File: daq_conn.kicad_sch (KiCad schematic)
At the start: 1 part

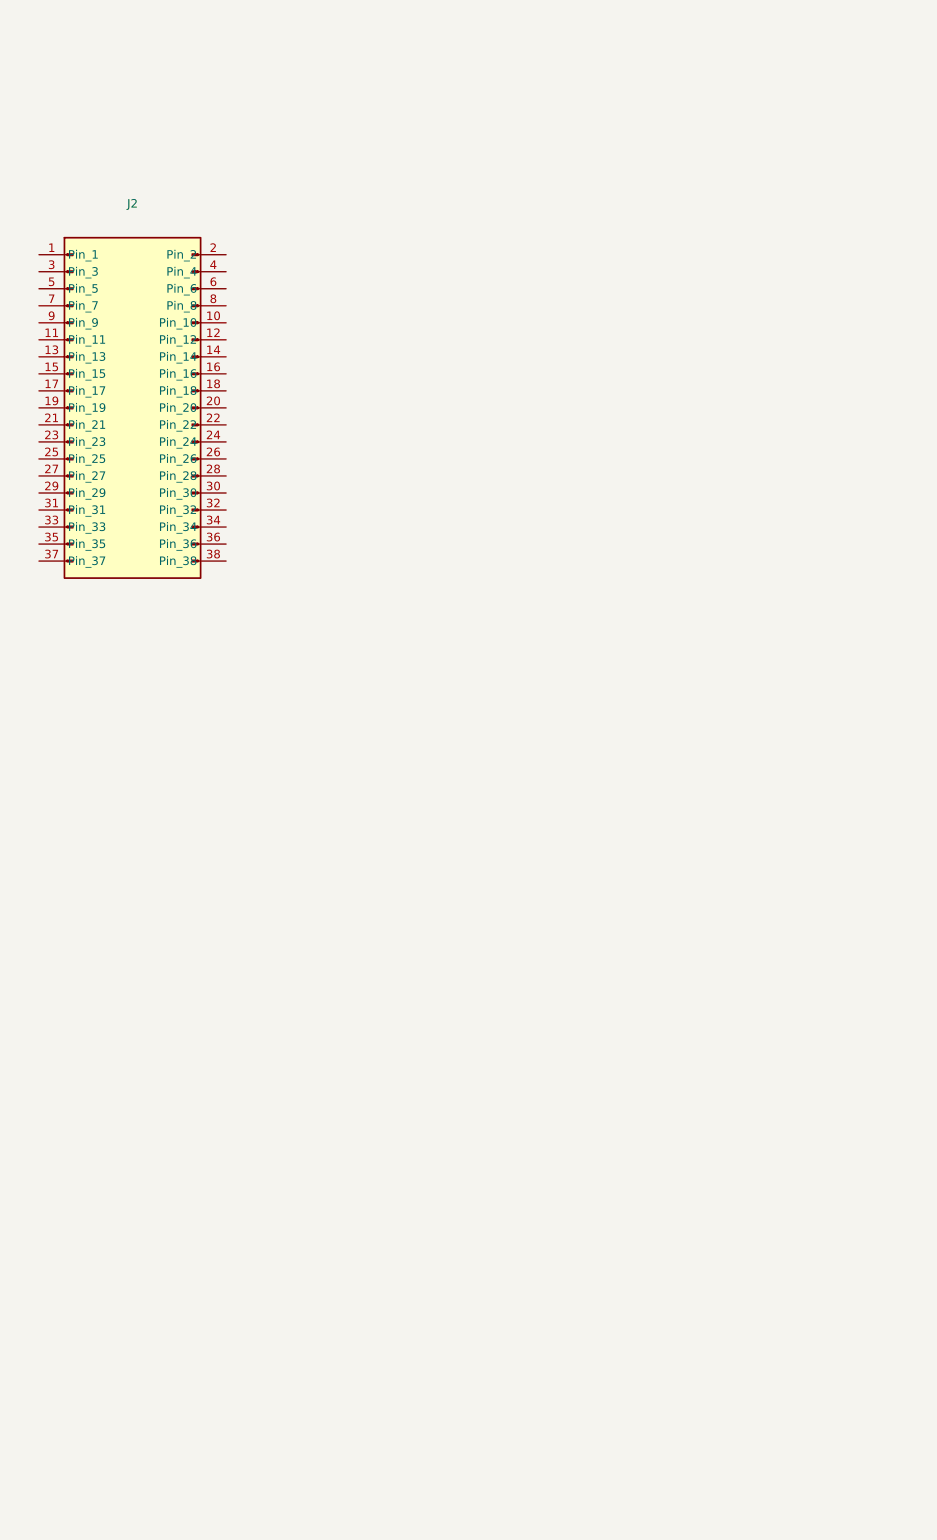
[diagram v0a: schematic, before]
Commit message: started on adc
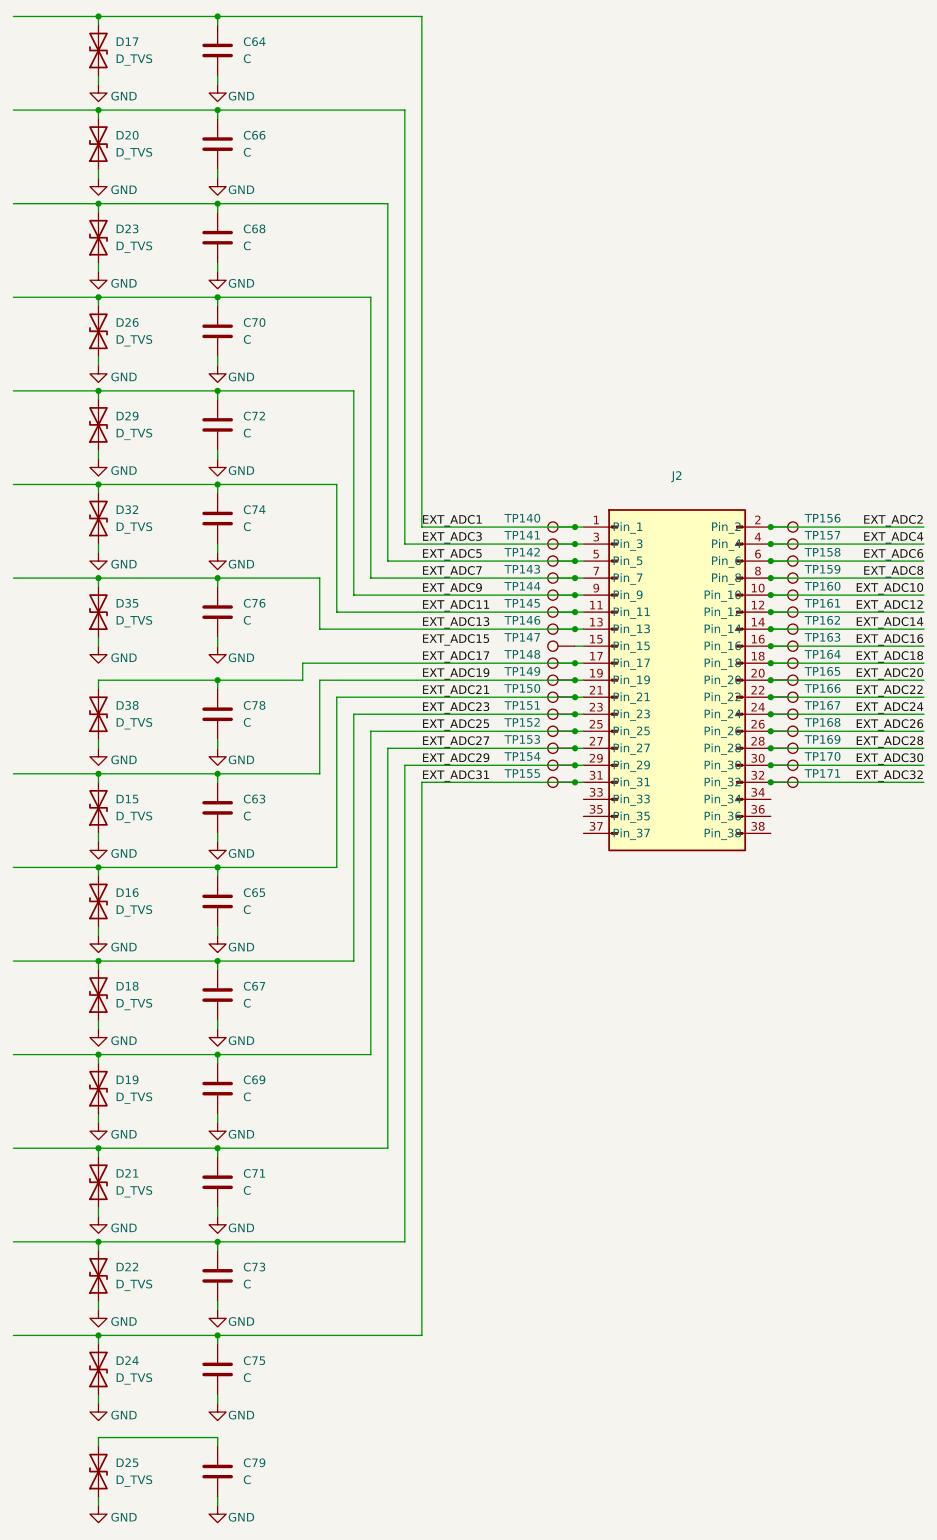
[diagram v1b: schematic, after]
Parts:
- added C63, C64, C65, C66, C67, C68, C69, C70, C71, C72, C73, C74, C75, C76, C78, C79: C, symbol Device:C
- added D15, D16, D17, D18, D19, D20, D21, D22, D23, D24, D25, D26, D29, D32, D35, D38: D_TVS, symbol Device:D_TVS
- added TP140, TP141, TP142, TP143, TP144, TP145, TP146, TP147, TP148, TP149, TP150, TP151, TP152, TP153, TP154, TP155, TP156, TP157, TP158, TP159, TP160, TP161, TP162, TP163, TP164, TP165, TP166, TP167, TP168, TP169, TP170, TP171: TestPoint, symbol Connector:TestPoint
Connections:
- net EXT_ADC1: now reaches J2.1 (Pin_1)
- net EXT_ADC1: now also C64.1, D17.2 (A2), TP140.1
- net EXT_ADC10: now reaches J2.10 (Pin_10)
- net EXT_ADC10: now also TP160.1
- net EXT_ADC11: now reaches J2.11 (Pin_11)
- net EXT_ADC11: now also C74.1, D32.2 (A2), TP145.1
- net EXT_ADC12: now reaches J2.12 (Pin_12)
- net EXT_ADC12: now also TP161.1
- net EXT_ADC13: now reaches J2.13 (Pin_13)
- net EXT_ADC13: now also C76.1, D35.2 (A2), TP146.1
- net EXT_ADC14: now reaches J2.14 (Pin_14)
- net EXT_ADC14: now also TP162.1
- net at J2.15 (Pin_15): now also TP147.1
- net EXT_ADC16: now reaches J2.16 (Pin_16)
- net EXT_ADC16: now also TP163.1
- net EXT_ADC17: now reaches J2.17 (Pin_17)
- net EXT_ADC17: now also C78.1, D38.2 (A2), TP148.1
- net EXT_ADC18: now reaches J2.18 (Pin_18)
- net EXT_ADC18: now also TP164.1
- net EXT_ADC19: now reaches J2.19 (Pin_19)
- net EXT_ADC19: now also C63.1, D15.2 (A2), TP149.1
- net EXT_ADC2: now reaches J2.2 (Pin_2)
- net EXT_ADC2: now also TP156.1
- net EXT_ADC20: now reaches J2.20 (Pin_20)
- net EXT_ADC20: now also TP165.1
- net EXT_ADC21: now reaches J2.21 (Pin_21)
- net EXT_ADC21: now also C65.1, D16.2 (A2), TP150.1
- net EXT_ADC22: now reaches J2.22 (Pin_22)
- net EXT_ADC22: now also TP166.1
- net EXT_ADC23: now reaches J2.23 (Pin_23)
- net EXT_ADC23: now also C67.1, D18.2 (A2), TP151.1
- net EXT_ADC24: now reaches J2.24 (Pin_24)
- net EXT_ADC24: now also TP167.1
- net EXT_ADC25: now reaches J2.25 (Pin_25)
- net EXT_ADC25: now also C69.1, D19.2 (A2), TP152.1
- net EXT_ADC26: now reaches J2.26 (Pin_26)
- net EXT_ADC26: now also TP168.1
- net EXT_ADC27: now reaches J2.27 (Pin_27)
- net EXT_ADC27: now also C71.1, D21.2 (A2), TP153.1
- net EXT_ADC28: now reaches J2.28 (Pin_28)
- net EXT_ADC28: now also TP169.1
- net EXT_ADC29: now reaches J2.29 (Pin_29)
- net EXT_ADC29: now also C73.1, D22.2 (A2), TP154.1
- net EXT_ADC3: now reaches J2.3 (Pin_3)
- net EXT_ADC3: now also C66.1, D20.2 (A2), TP141.1
- net EXT_ADC30: now reaches J2.30 (Pin_30)
- net EXT_ADC30: now also TP170.1
- net EXT_ADC31: now reaches J2.31 (Pin_31)
- net EXT_ADC31: now also C75.1, D24.2 (A2), TP155.1
- net EXT_ADC32: now reaches J2.32 (Pin_32)
- net EXT_ADC32: now also TP171.1
- net EXT_ADC4: now reaches J2.4 (Pin_4)
- net EXT_ADC4: now also TP157.1
- net EXT_ADC5: now reaches J2.5 (Pin_5)
- net EXT_ADC5: now also C68.1, D23.2 (A2), TP142.1
- net EXT_ADC6: now reaches J2.6 (Pin_6)
- net EXT_ADC6: now also TP158.1
- net EXT_ADC7: now reaches J2.7 (Pin_7)
- net EXT_ADC7: now also C70.1, D26.2 (A2), TP143.1
- net EXT_ADC8: now reaches J2.8 (Pin_8)
- net EXT_ADC8: now also TP159.1
- net EXT_ADC9: now reaches J2.9 (Pin_9)
- net EXT_ADC9: now also C72.1, D29.2 (A2), TP144.1
- new net: C79.1, D25.2 (A2)
- new net GND: C63.2, C64.2, C65.2, C66.2, C67.2, C68.2, C69.2, C70.2, C71.2, C72.2, C73.2, C74.2, C75.2, C76.2, C78.2, C79.2, D15.1 (A1), D16.1 (A1), D17.1 (A1), D18.1 (A1), D19.1 (A1), D20.1 (A1), D21.1 (A1), D22.1 (A1), D23.1 (A1), D24.1 (A1), D25.1 (A1), D26.1 (A1), D29.1 (A1), D32.1 (A1), D35.1 (A1), D38.1 (A1)
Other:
- moved on the sheet: J2
